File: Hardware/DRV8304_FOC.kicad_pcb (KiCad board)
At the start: 4 copper layers, 61 x 61 mm, 75 parts, among them J1 Conn_01x01_Pin, J2 Conn_01x01_Pin, J3 Conn_01x01_Pin, J6 Conn_01x01_Pin, J7 Conn_01x01_Pin, J8 Conn_01x01_Pin, J9 TC2070, Q1 SIRA18ADP, Q2 SIRA18ADP, Q3 SIRA18ADP, Q4 SIRA18ADP, Q5 SIRA18ADP, Q6 SIRA18ADP, SW2 SW_Push, U1 TPS565208, U3 DRV8304HRHAR, U4 STM32F412CEUx, U6 AS5047P, Y1 Crystal_GND23

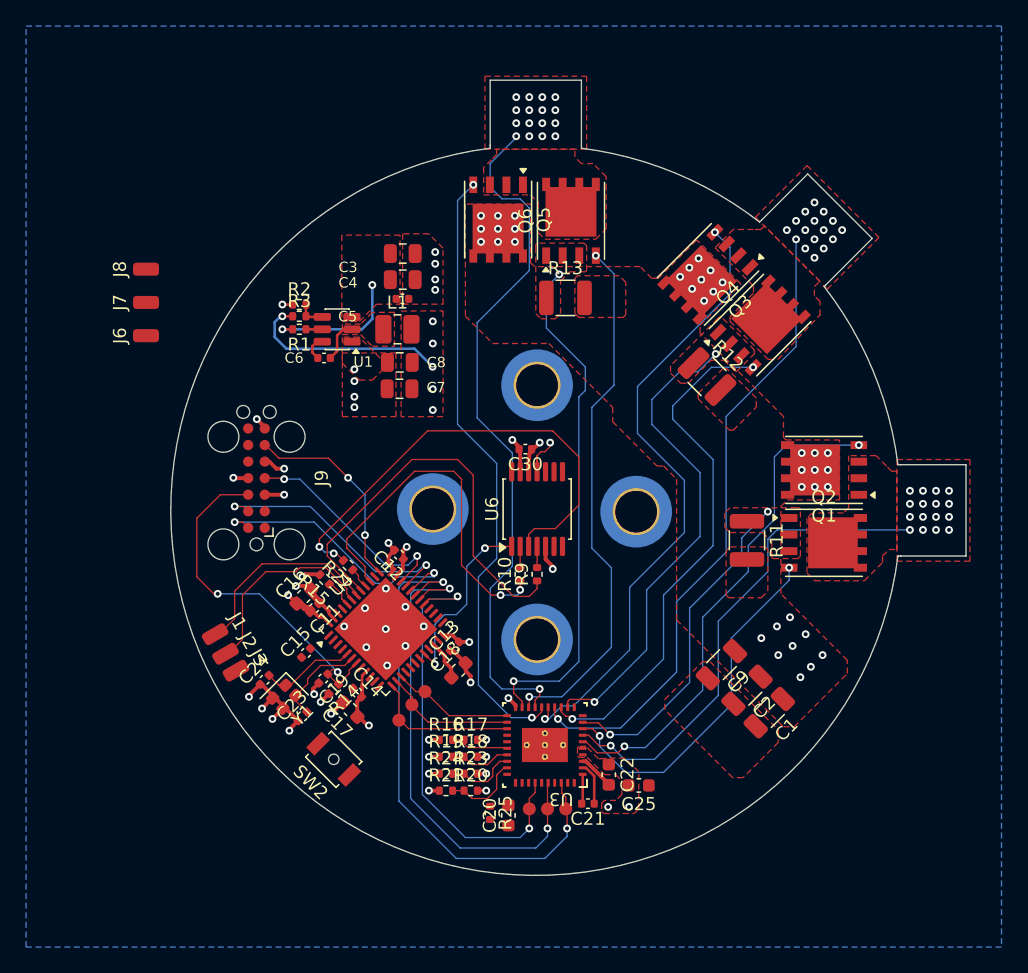
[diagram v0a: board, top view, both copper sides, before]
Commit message: Commit for review
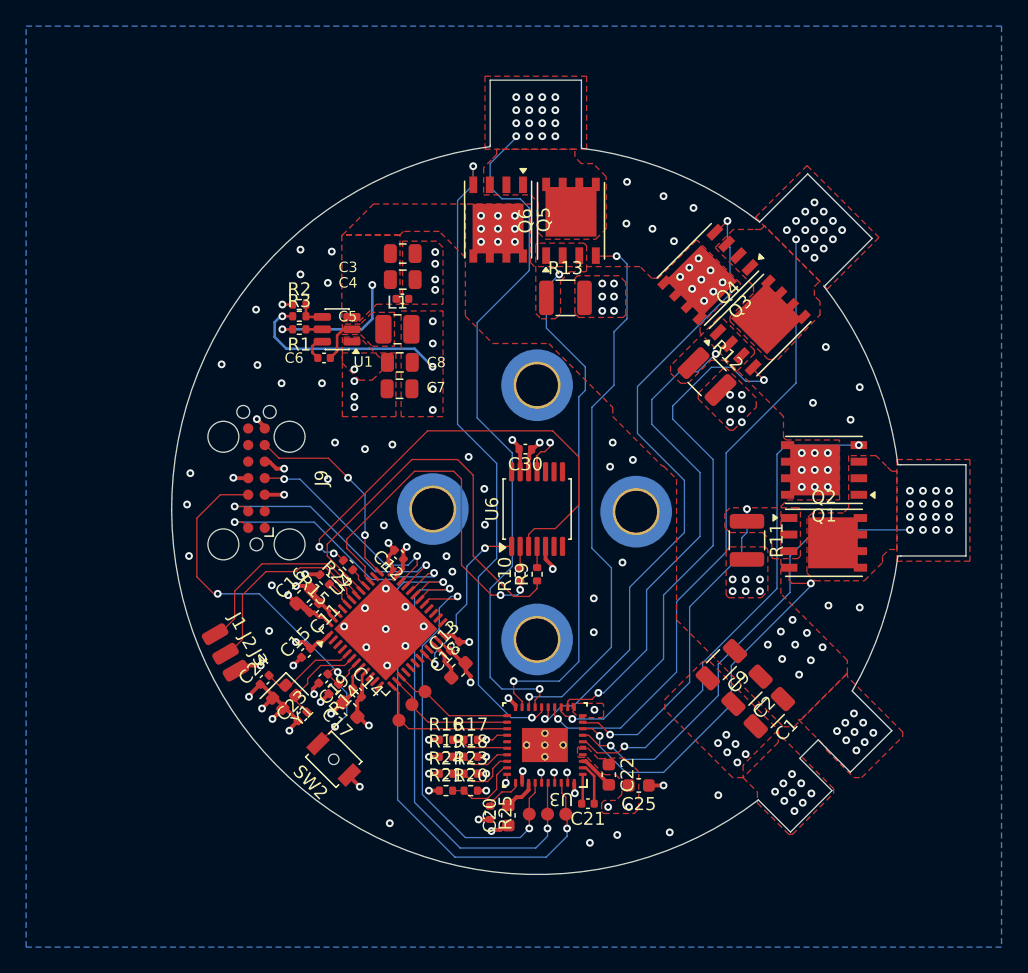
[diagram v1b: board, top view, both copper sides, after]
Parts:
- removed J6, J7, J8: Conn_01x01_Pin, Connector_Wire:SolderWirePad_1x01_SMD_1x2mm
- moved TP1 0.40 mm to (152.5, 127.6)
- moved TP3 0.40 mm to (153.9, 127.6)
- moved TP5 0.40 mm to (155.3, 127.6)
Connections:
- U3 pad V: (no net) -> GND
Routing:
- net GND: track 36.0 -> 49.7 mm, vias 38 -> 127
- net 3V3: track 41.6 -> 49.7 mm, vias 18 -> 23
- net /~{RST}: track 27.3 -> 34.0 mm, vias 2 -> 3
- net Net-(U3-CAL): track 0.00 -> 3.01 mm
- net GHC: track 47.1 -> 50.0 mm
- net GLB: track 40.0 -> 42.6 mm
- net Net-(U3-DVDD): track 0.00 -> 2.59 mm
- net GLA: track 27.8 -> 30.0 mm
- net GLC: track 40.6 -> 42.5 mm
- net GHB: track 48.4 -> 50.2 mm
- net SHA: track 38.0 -> 36.2 mm
- net INHC: track 33.9 -> 33.3 mm
- net SPI_~{SS}: track 14.3 -> 13.8 mm
- net Vin: vias 40 -> 49
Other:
- board size 61 x 61 mm -> 60.9 x 60.9 mm

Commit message: FAB OUT GERBER
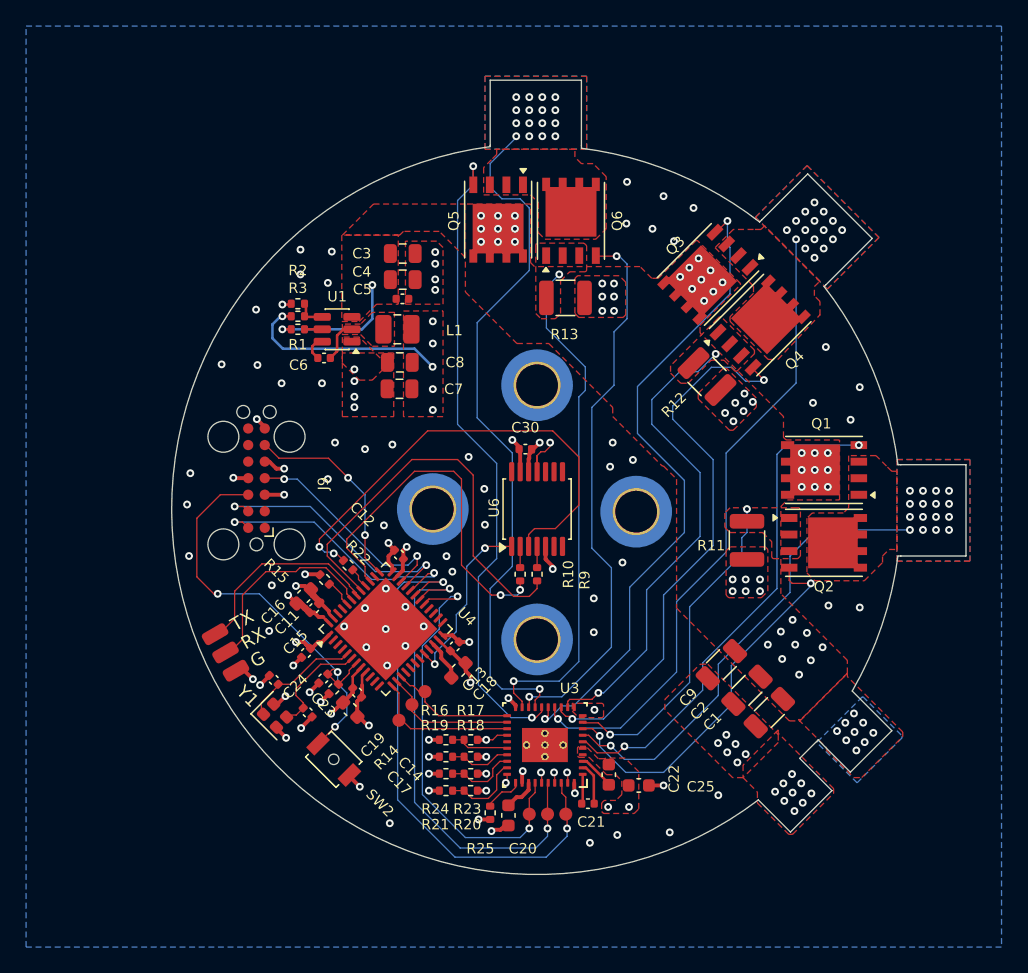
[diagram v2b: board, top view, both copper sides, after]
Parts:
- Y1: value Crystal_GND23 -> Crystal_GND24
- moved Y1 1.61 mm to (133.0, 120.0), turned to -45 degrees
- moved C24 0.70 mm to (132.9, 117.3), turned to -45 degrees
- moved C23 0.50 mm to (135.5, 119.8), turned to 135 degrees
- moved R2 0.13 mm to (134.8, 88.4)
- moved R1 0.11 mm to (134.8, 90.4)
- moved R3 0.11 mm to (134.8, 89.4)
- moved J2 0.10 mm to (129.2, 115.2)
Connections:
- Y1 pad 3: GND -> Net-(U4-PH1)
- Y1 pad 4: Net-(U4-PH1) -> GND
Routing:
- net GND: track 49.7 -> 44.7 mm
- net Net-(U4-PH0): track 7.30 -> 9.17 mm
- net Net-(U4-PH1): track 7.33 -> 8.51 mm
- added copper zone on B.Cu, net SHA
- added copper zone on B.Cu, net SHB
- added copper zone on B.Cu, net SHC
- added copper zone on B.Cu, net Vin
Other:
- board text added: "G"
- board text added: "RX"
- board text added: "TX"
